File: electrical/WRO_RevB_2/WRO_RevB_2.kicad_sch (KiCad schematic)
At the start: 22 parts, among them J11 MOTOR, J2 Conn_01x04_Pin, J3 Conn_01x04_Pin, J4 Conn_01x11_Pin, J5 Conn_01x08_Pin, U2 ROB-14450

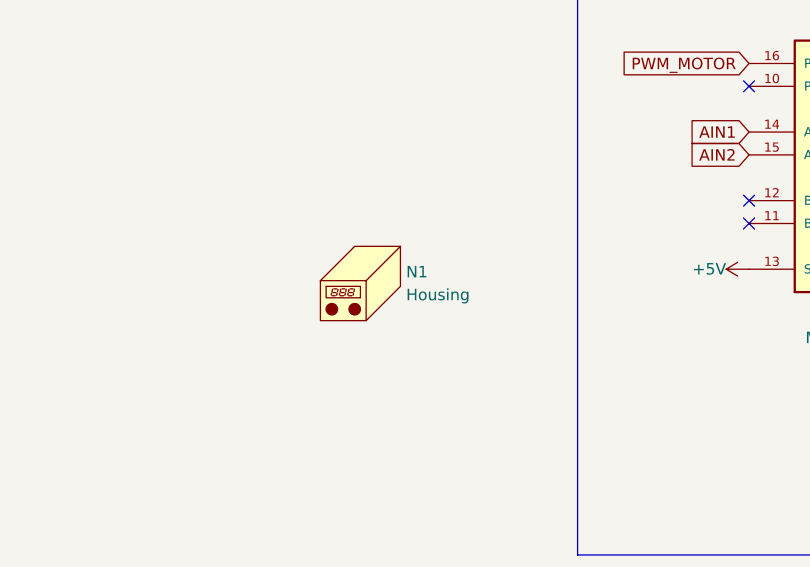
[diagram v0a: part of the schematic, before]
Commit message: Revert "Merge branch 'main' of https://github.com/Nakashima26/WRO_FE_2026_FoxRobotics"
This reverts commit 232f9ecb01216201165b5abf43ae09e229c3eea8, reversing
changes made to 212c0f9856f89e84f48e320d89d4fd8fc24ab9e3.
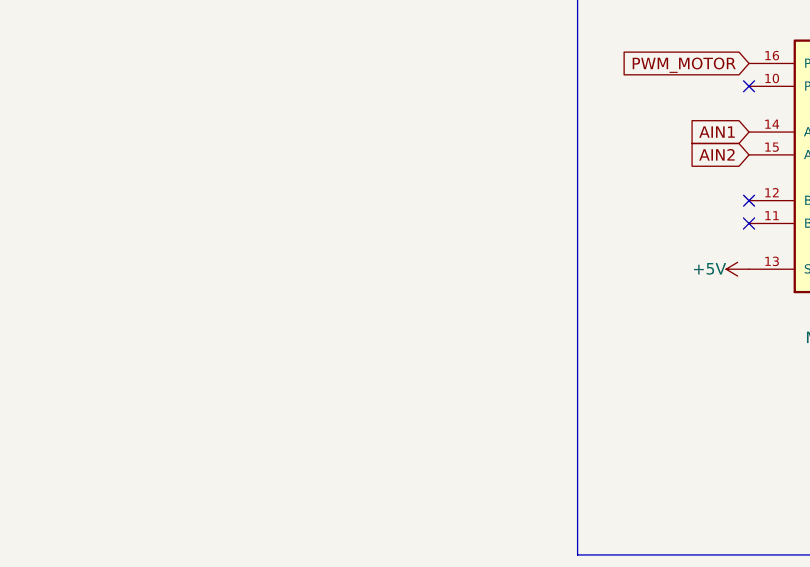
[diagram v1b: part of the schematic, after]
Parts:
- removed N1: Housing, Symbol:KiCad-Logo2_12mm_SilkScreen, symbol Mechanical:Housing
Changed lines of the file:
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@@
-	)
-	(symbol
-		(lib_id "Mechanical:Housing")
-		(at 78.74 137.16 0)
-		(unit 1)
-		(body_style 1)
-		(exclude_from_sim no)
-		(in_bom yes)
-		(on_board yes)
-		(in_pos_files yes)
-		(dnp no)
-		(fields_autoplaced yes)
-		(property "Reference" "N1"
-			(at 82.55 136.2074 0)
-			(show_name no)
-			(do_not_autoplace no)
-			(effects
-				(font
-					(size 1.27 1.27)
-				)
-				(justify left)
-			)
-		)
-		(property "Value" "Housing"
-			(at 82.55 138.7474 0)
-			(show_name no)
-			(do_not_autoplace no)
-			(effects
-				(font
-					(size 1.27 1.27)
-				)
-				(justify left)
-			)
-		)
-		(property "Footprint" "Symbol:KiCad-Logo2_12mm_SilkScreen"
-			(at 80.01 135.89 0)
-			(hide yes)
-			(show_name no)
-			(do_not_autoplace no)
-			(effects
-				(font
-					(size 1.27 1.27)
-				)
-			)
-		)
-		(property "Datasheet" ""
-			(at 80.01 135.89 0)
-			(hide yes)
-			(show_name no)
-			(do_not_autoplace no)
-			(effects
-				(font
-					(size 1.27 1.27)
-				)
-			)
-		)
-		(property "Description" "Housing"
-			(at 78.74 137.16 0)
-			(hide yes)
-			(show_name no)
-			(do_not_autoplace no)
-			(effects
-				(font
-					(size 1.27 1.27)
-				)
-			)
-		)
-		(instances
-			(project "WRO_RevB_2"
-				(path "/1b47eb32-0907-4bd9-a4c8-0f6808dfb617"
-					(reference "N1")
-					(unit 1)
-				)
-			)
-		)
 	)
 	(symbol

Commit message: actualiza PCB RevB
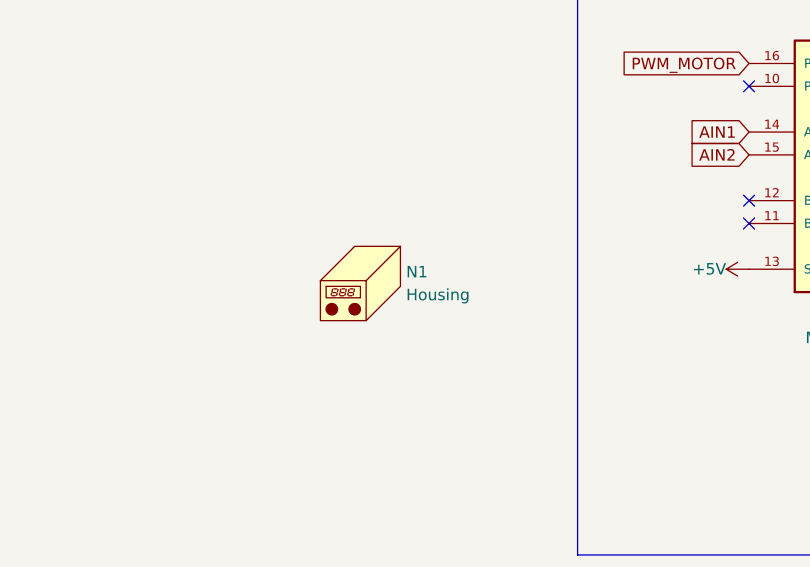
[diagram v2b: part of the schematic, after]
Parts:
- added N1: Housing, Symbol:KiCad-Logo2_12mm_SilkScreen, symbol Mechanical:Housing
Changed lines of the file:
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@@
+	)
+	(symbol
+		(lib_id "Mechanical:Housing")
+		(at 78.74 137.16 0)
+		(unit 1)
+		(body_style 1)
+		(exclude_from_sim no)
+		(in_bom yes)
+		(on_board yes)
+		(in_pos_files yes)
+		(dnp no)
+		(fields_autoplaced yes)
+		(property "Reference" "N1"
+			(at 82.55 136.2074 0)
+			(show_name no)
+			(do_not_autoplace no)
+			(effects
+				(font
+					(size 1.27 1.27)
+				)
+				(justify left)
+			)
+		)
+		(property "Value" "Housing"
+			(at 82.55 138.7474 0)
+			(show_name no)
+			(do_not_autoplace no)
+			(effects
+				(font
+					(size 1.27 1.27)
+				)
+				(justify left)
+			)
+		)
+		(property "Footprint" "Symbol:KiCad-Logo2_12mm_SilkScreen"
+			(at 80.01 135.89 0)
+			(hide yes)
+			(show_name no)
+			(do_not_autoplace no)
+			(effects
+				(font
+					(size 1.27 1.27)
+				)
+			)
+		)
+		(property "Datasheet" ""
+			(at 80.01 135.89 0)
+			(hide yes)
+			(show_name no)
+			(do_not_autoplace no)
+			(effects
+				(font
+					(size 1.27 1.27)
+				)
+			)
+		)
+		(property "Description" "Housing"
+			(at 78.74 137.16 0)
+			(hide yes)
+			(show_name no)
+			(do_not_autoplace no)
+			(effects
+				(font
+					(size 1.27 1.27)
+				)
+			)
+		)
+		(instances
+			(project "WRO_RevB_2"
+				(path "/1b47eb32-0907-4bd9-a4c8-0f6808dfb617"
+					(reference "N1")
+					(unit 1)
+				)
+			)
+		)
 	)
 	(symbol

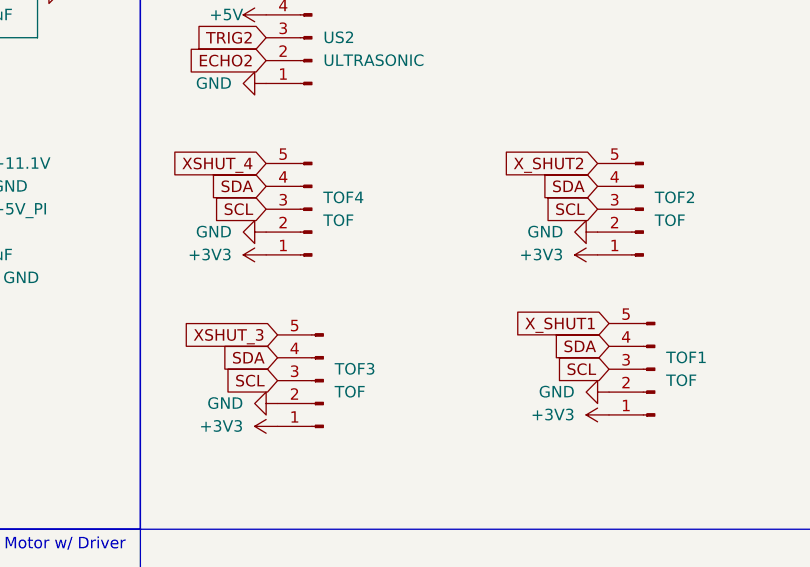
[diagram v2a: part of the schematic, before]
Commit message: pcb done (again)
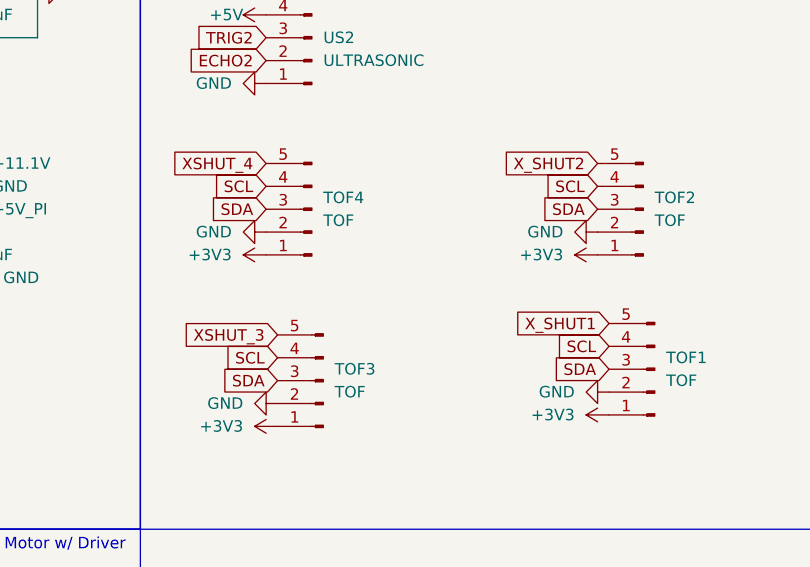
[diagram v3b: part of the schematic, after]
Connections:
- net SCL: now also TOF1.4 (Pin_4), TOF2.4 (Pin_4), TOF3.4 (Pin_4), TOF4.4 (Pin_4); no longer TOF1.3 (Pin_3), TOF2.3 (Pin_3), TOF3.3 (Pin_3), TOF4.3 (Pin_3)
- net SDA: now also TOF1.3 (Pin_3), TOF2.3 (Pin_3), TOF3.3 (Pin_3), TOF4.3 (Pin_3); no longer TOF1.4 (Pin_4), TOF2.4 (Pin_4), TOF3.4 (Pin_4), TOF4.4 (Pin_4)
